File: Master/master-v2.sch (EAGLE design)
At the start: 59 parts, among them J1 ISP, K1 653002114822, K2 653002114822, K3 653002114822, K4 653002114822, U1 ATMEGA128RFA1, U3 ULN2003ANE4, Y1 16MHz, Y2 32.768kHz

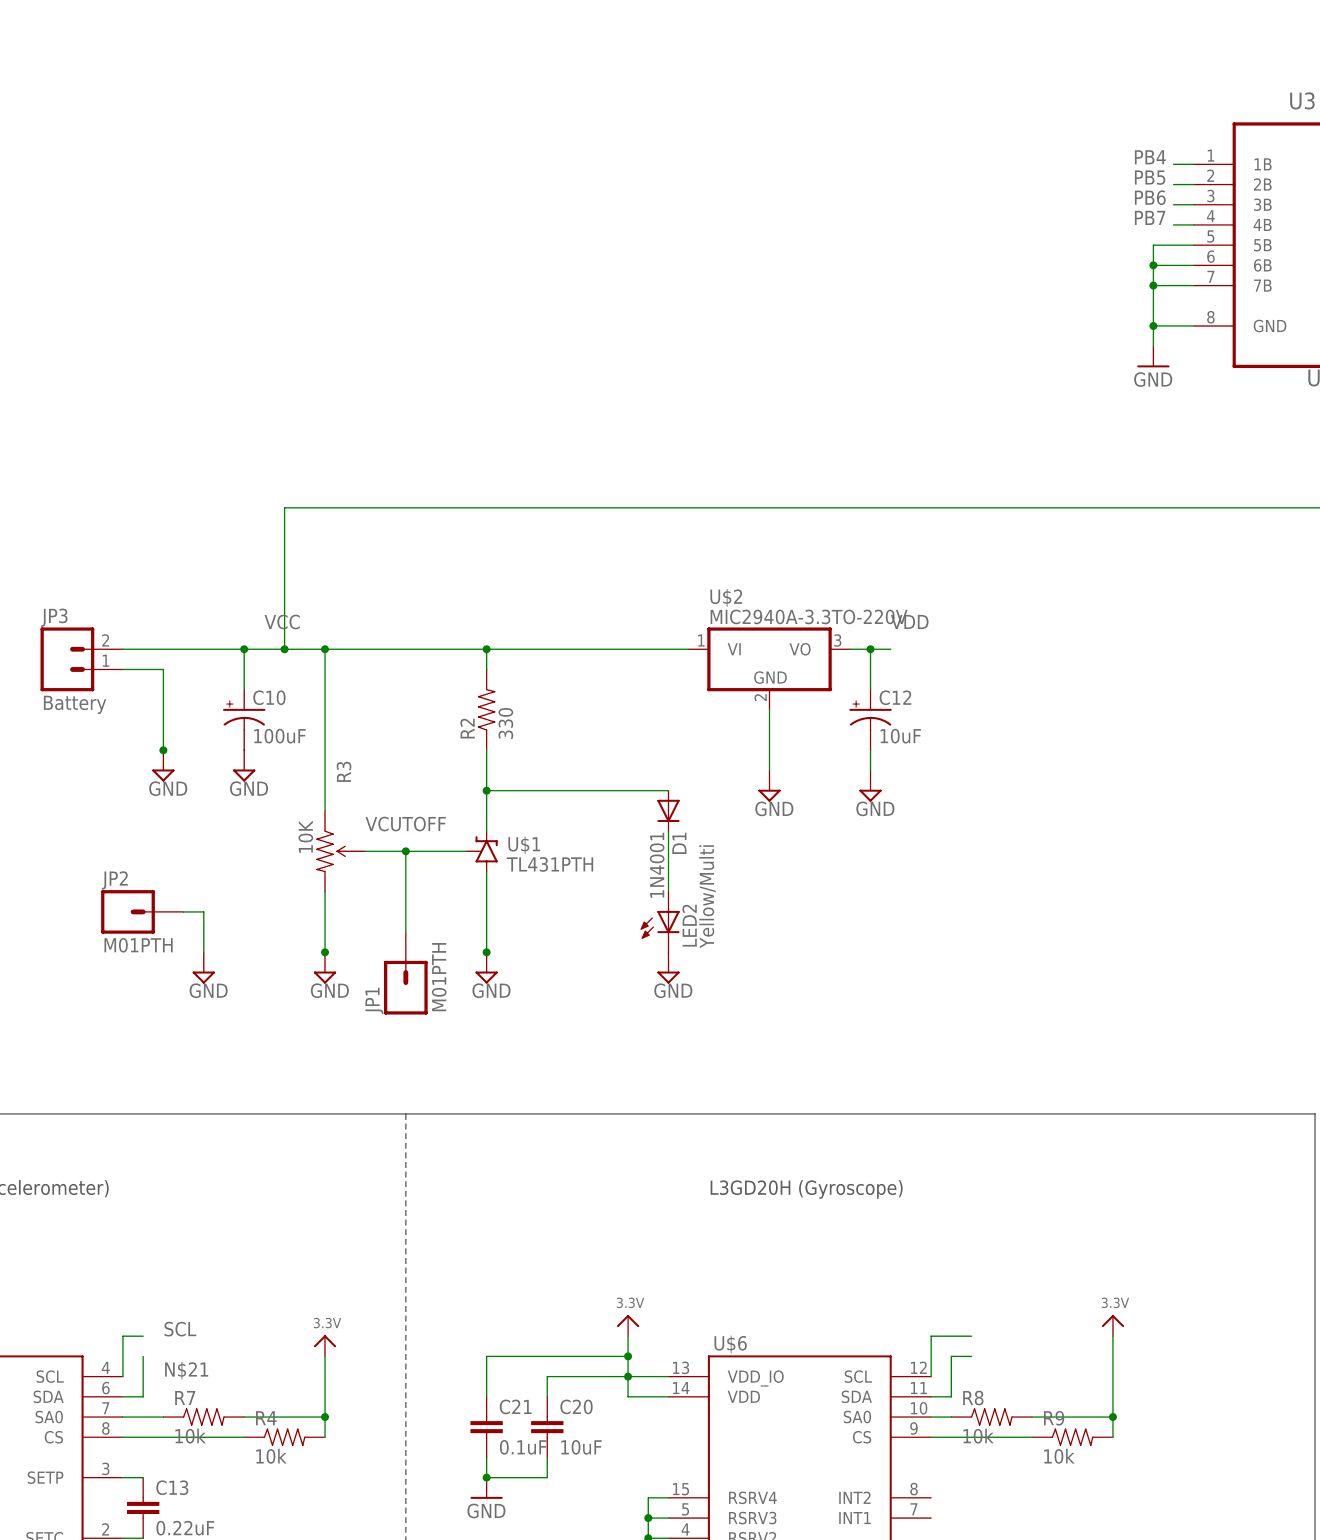
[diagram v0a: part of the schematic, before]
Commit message: changes to master-v2
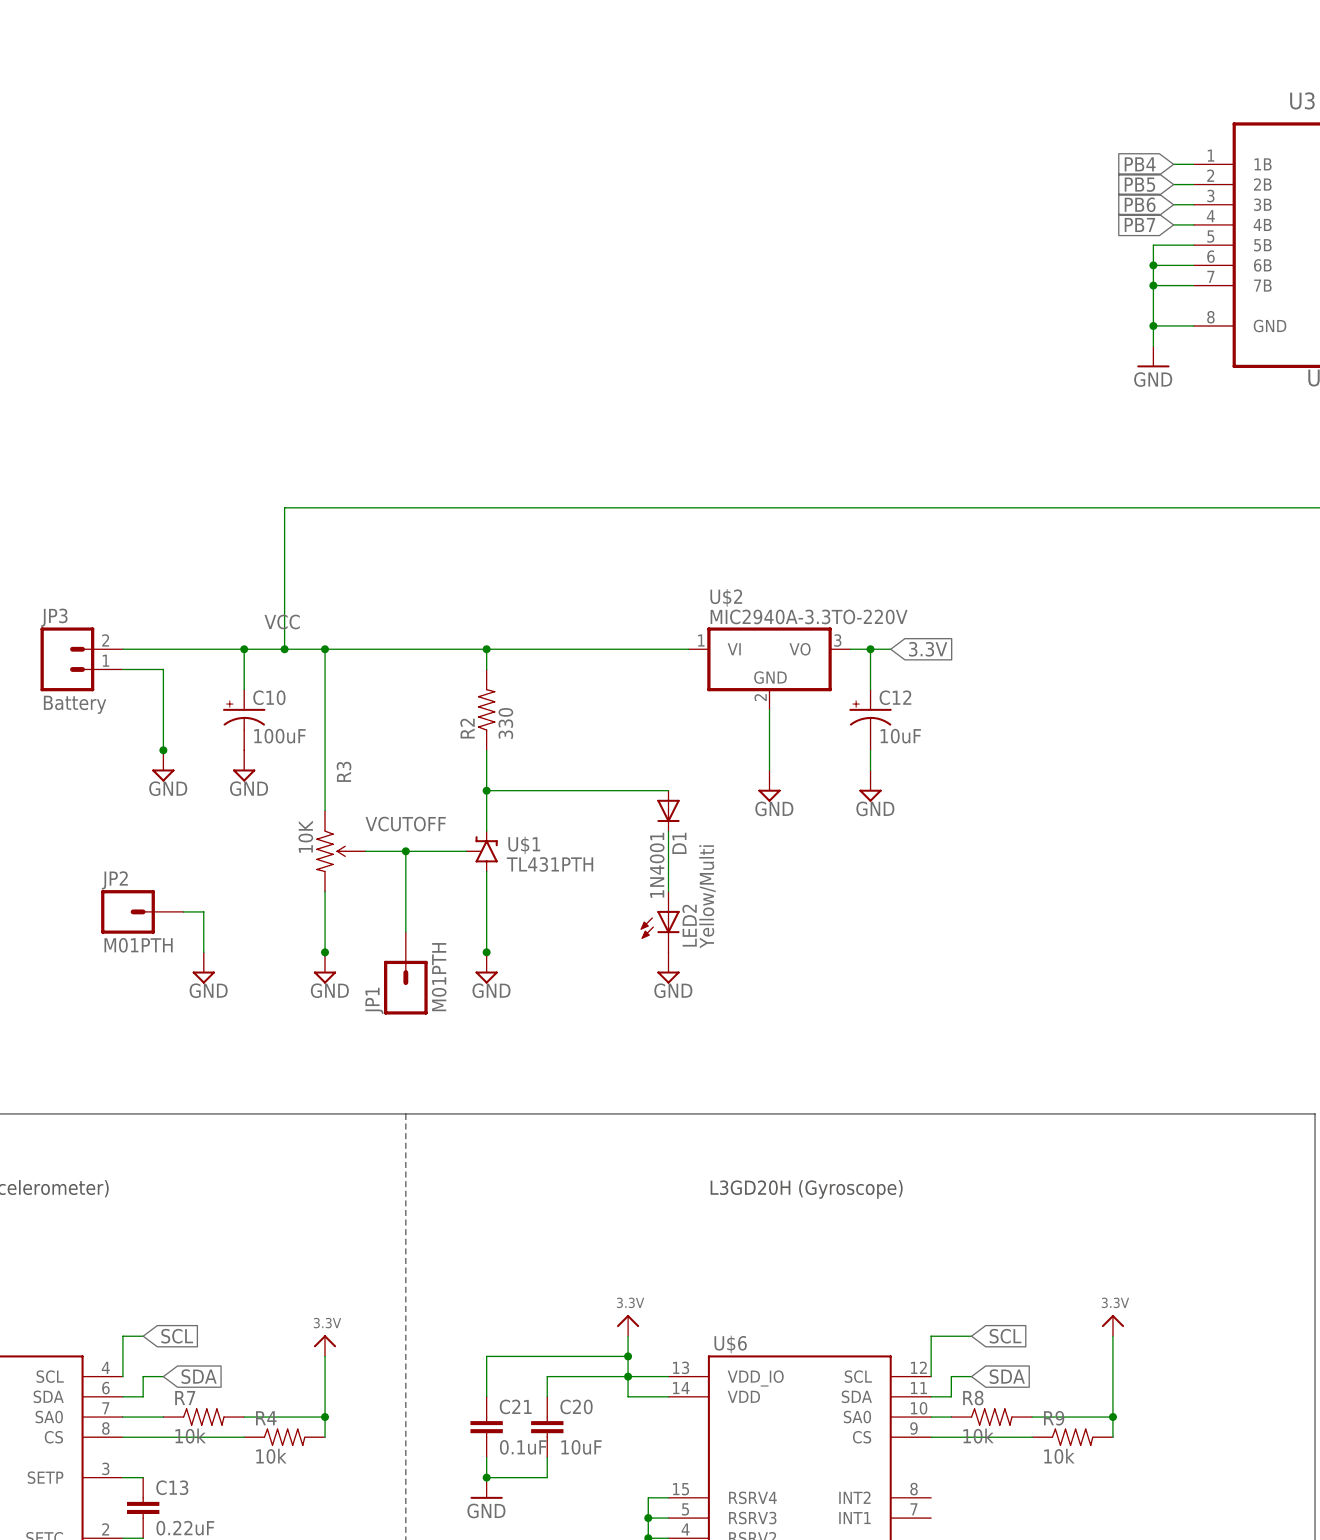
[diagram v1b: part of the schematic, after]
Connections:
- removed net N$21: U$3.SDA
- removed net N$22: U$6.SCL
- removed net N$23: U$6.SDA
- removed net VDD: C12.+, U$2.VO
- net 3.3V: now also C12.+, U$2.VO
- net SCL: now also U$6.SCL
- net SDA: now also U$3.SDA, U$6.SDA
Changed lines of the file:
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@@
 <label x="-5.08" y="99.06" size="1.27" layer="95" rot="MR0" xref="yes"/>
+</segment>
+<segment>
+<pinref part="U$3" gate="G$1" pin="SDA"/>
+<wire x1="-213.36" y1="78.74" x2="-210.82" y2="78.74" width="0.1524" layer="91"/>
+<wire x1="-210.82" y1="78.74" x2="-210.82" y2="81.28" width="0.1524" layer="91"/>
+<wire x1="-210.82" y1="81.28" x2="-208.28" y2="81.28" width="0.1524" layer="91"/>
+<label x="-208.28" y="81.28" size="1.778" layer="95" xref="yes"/>
+</segment>
+<segment>
+<pinref part="U$6" gate="G$1" pin="SDA"/>
+<wire x1="-111.76" y1="78.74" x2="-109.22" y2="78.74" width="0.1524" layer="91"/>
+<wire x1="-109.22" y1="78.74" x2="-109.22" y2="81.28" width="0.1524" layer="91"/>
+<wire x1="-109.22" y1="81.28" x2="-106.68" y2="81.28" width="0.1524" layer="91"/>
+<label x="-106.68" y="81.28" size="1.778" layer="95" xref="yes"/>
 </segment>
 </net>
@@
 <wire x1="-213.36" y1="81.28" x2="-213.36" y2="86.36" width="0.1524" layer="91"/>
 <wire x1="-213.36" y1="86.36" x2="-210.82" y2="86.36" width="0.1524" layer="91"/>
-<label x="-208.28" y="86.36" size="1.778" layer="95"/>
+<label x="-210.82" y="86.36" size="1.778" layer="95" xref="yes"/>
+</segment>
+<segment>
+<pinref part="U$6" gate="G$1" pin="SCL"/>
+<wire x1="-111.76" y1="81.28" x2="-111.76" y2="86.36" width="0.1524" layer="91"/>
+<wire x1="-111.76" y1="86.36" x2="-106.68" y2="86.36" width="0.1524" layer="91"/>
+<label x="-106.68" y="86.36" size="1.778" layer="95" xref="yes"/>
 </segment>
 </net>
@@
 <pinref part="U3" gate="A" pin="4B"/>
 <wire x1="-78.74" y1="226.06" x2="-81.28" y2="226.06" width="0.1524" layer="91"/>
-<label x="-86.36" y="226.06" size="1.778" layer="95"/>
+<label x="-81.28" y="226.06" size="1.778" layer="95" rot="R180" xref="yes"/>
 </segment>
 </net>
@@
 <pinref part="U3" gate="A" pin="3B"/>
 <wire x1="-78.74" y1="228.6" x2="-81.28" y2="228.6" width="0.1524" layer="91"/>
-<label x="-86.36" y="228.6" size="1.778" layer="95"/>
+<label x="-81.28" y="228.6" size="1.778" layer="95" rot="R180" xref="yes"/>
 </segment>
 </net>
@@
 <pinref part="U3" gate="A" pin="2B"/>
 <wire x1="-78.74" y1="231.14" x2="-81.28" y2="231.14" width="0.1524" layer="91"/>
-<label x="-86.36" y="231.14" size="1.778" layer="95"/>
+<label x="-81.28" y="231.14" size="1.778" layer="95" rot="R180" xref="yes"/>
 </segment>
 </net>
@@
 <pinref part="U3" gate="A" pin="1B"/>
 <wire x1="-78.74" y1="233.68" x2="-81.28" y2="233.68" width="0.1524" layer="91"/>
-<label x="-86.36" y="233.68" size="1.778" layer="95"/>
+<label x="-81.28" y="233.68" size="1.778" layer="95" rot="R180" xref="yes"/>
 </segment>
 </net>
@@
 <wire x1="-99.06" y1="76.2" x2="-88.9" y2="76.2" width="0.1524" layer="91"/>
 <junction x="-88.9" y="76.2"/>
+</segment>
+<segment>
+<pinref part="U$2" gate="G$1" pin="VO"/>
+<wire x1="-121.92" y1="172.72" x2="-119.38" y2="172.72" width="0.1524" layer="91"/>
+<pinref part="C12" gate="G$1" pin="+"/>
+<wire x1="-119.38" y1="172.72" x2="-116.84" y2="172.72" width="0.1524" layer="91"/>
+<wire x1="-119.38" y1="167.64" x2="-119.38" y2="172.72" width="0.1524" layer="91"/>
+<junction x="-119.38" y="172.72"/>
+<label x="-116.84" y="172.72" size="1.778" layer="95" xref="yes"/>
 </segment>
 </net>
@@
 </segment>
 </net>
-<net name="VDD" class="0">
-<segment>
-<pinref part="U$2" gate="G$1" pin="VO"/>
-<wire x1="-121.92" y1="172.72" x2="-119.38" y2="172.72" width="0.1524" layer="91"/>
-<label x="-116.84" y="175.26" size="1.778" layer="95"/>
-<pinref part="C12" gate="G$1" pin="+"/>
-<wire x1="-119.38" y1="172.72" x2="-116.84" y2="172.72" width="0.1524" layer="91"/>
-<wire x1="-119.38" y1="167.64" x2="-119.38" y2="172.72" width="0.1524" layer="91"/>
-<junction x="-119.38" y="172.72"/>
-</segment>
-</net>
 <net name="N$1" class="0">
 <segment>
@@
 </segment>
 </net>
-<net name="N$21" class="0">
-<segment>
-<pinref part="U$3" gate="G$1" pin="SDA"/>
-<wire x1="-213.36" y1="78.74" x2="-210.82" y2="78.74" width="0.1524" layer="91"/>
-<wire x1="-210.82" y1="78.74" x2="-210.82" y2="83.82" width="0.1524" layer="91"/>
-<label x="-208.28" y="81.28" size="1.778" layer="95"/>
-</segment>
-</net>
-<net name="N$22" class="0">
-<segment>
-<pinref part="U$6" gate="G$1" pin="SCL"/>
-<wire x1="-111.76" y1="81.28" x2="-111.76" y2="86.36" width="0.1524" layer="91"/>
-<wire x1="-111.76" y1="86.36" x2="-106.68" y2="86.36" width="0.1524" layer="91"/>
-</segment>
-</net>
-<net name="N$23" class="0">
-<segment>
-<pinref part="U$6" gate="G$1" pin="SDA"/>
-<wire x1="-111.76" y1="78.74" x2="-109.22" y2="78.74" width="0.1524" layer="91"/>
-<wire x1="-109.22" y1="78.74" x2="-109.22" y2="83.82" width="0.1524" layer="91"/>
-<wire x1="-109.22" y1="83.82" x2="-106.68" y2="83.82" width="0.1524" layer="91"/>
-</segment>
-</net>
